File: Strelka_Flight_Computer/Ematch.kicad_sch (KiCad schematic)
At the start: 11 parts, among them Q10 AP2300, Q11 MMBT2222, Q9 AO3401A

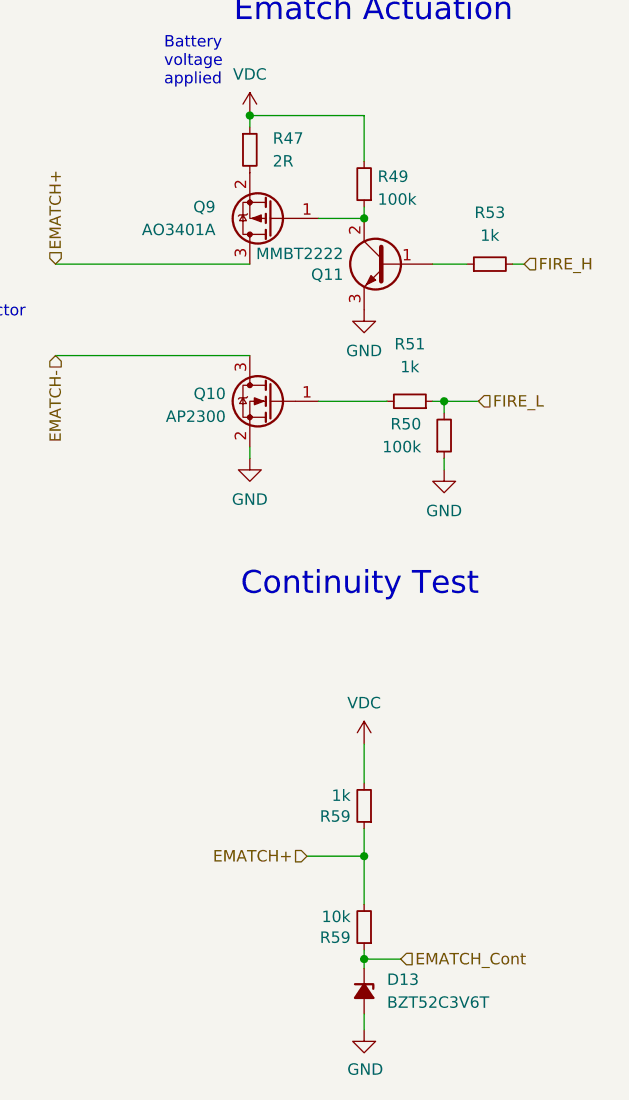
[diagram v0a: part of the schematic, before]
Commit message: Routing starting
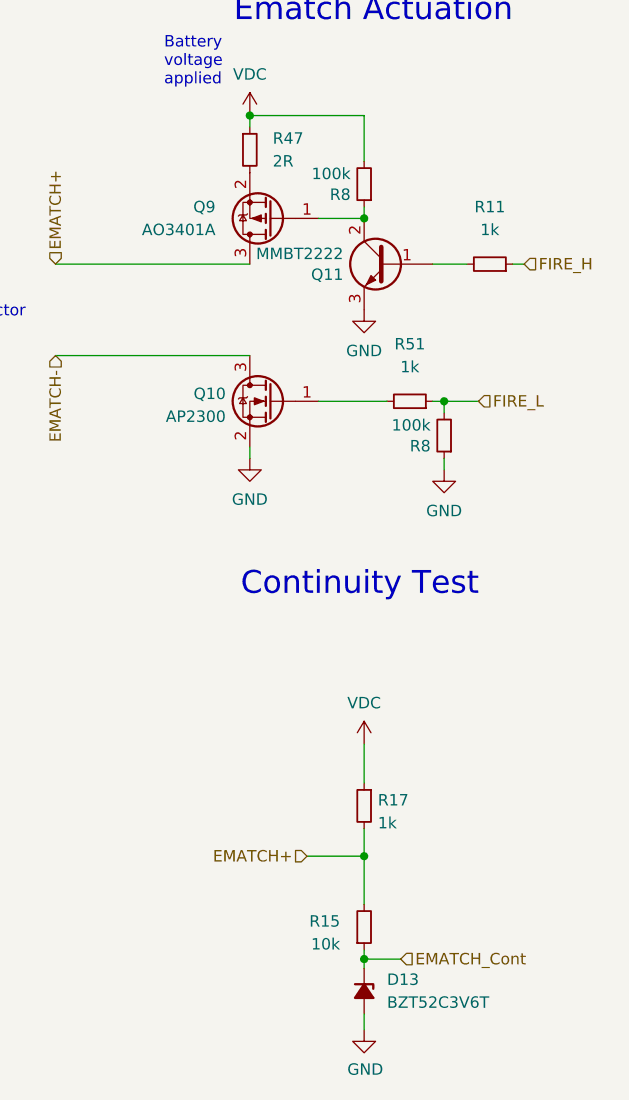
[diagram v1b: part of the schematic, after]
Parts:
- removed R49, R50: 100k, Resistor_SMD:R_0603_1608Metric, symbol Device:R_Small
- removed R53, R59: 1k, Resistor_SMD:R_0603_1608Metric, symbol Device:R_Small
- removed R59: 10k, Resistor_SMD:R_0603_1608Metric, symbol Device:R_Small
- added R11, R17: 1k, Resistor_SMD:R_0402_1005Metric, symbol Device:R_Small
- added R15: 10k, Resistor_SMD:R_0402_1005Metric, symbol Device:R_Small
- added R8 (x2): 100k, Resistor_SMD:R_0402_1005Metric, symbol Device:R_Small
- R51: footprint Resistor_SMD:R_0603_1608Metric -> Resistor_SMD:R_0402_1005Metric; LCSC (none) -> C11702
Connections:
- net EMATCH+: now also R15.2, R17.2
- net EMATCH_Cont: now also R15.1
- net FIRE_H: now also R11.1
- net FIRE_L: now also R8.2
- net GND: now also R8.1
- net VDC: now also R17.1, R8.2
- net at Q11.2 (C), Q9.1 (G): now also R8.1
- net at Q11.1 (B): now also R11.2

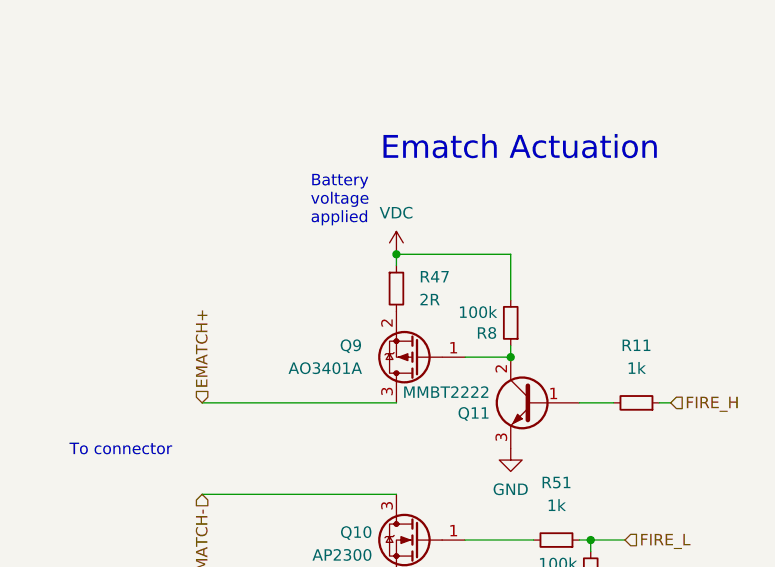
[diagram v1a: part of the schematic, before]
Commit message: Routing complete
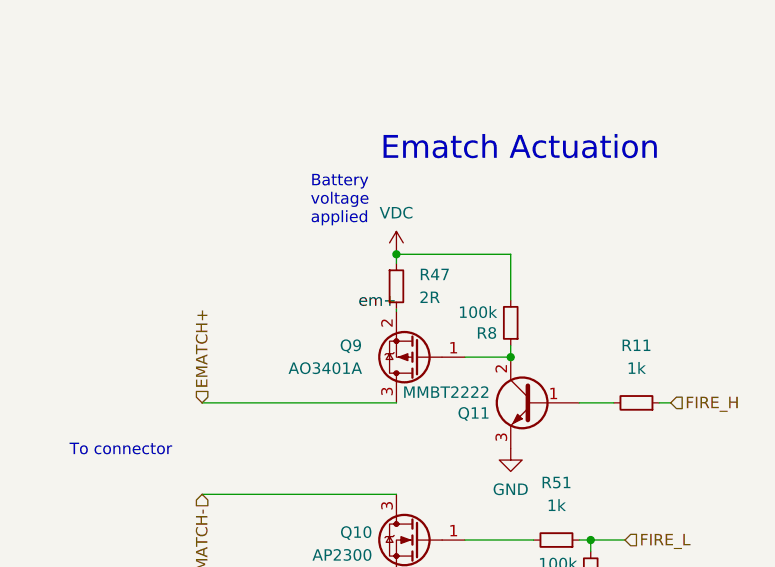
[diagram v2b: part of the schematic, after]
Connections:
- net em+: now reaches Q9.2 (S), R47.2
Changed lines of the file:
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@@
     (stroke (width 0) (type default))
   )
-  (wire (pts (xy 127 43.18) (xy 127 44.45))
+  (wire (pts (xy 127 49.276) (xy 127 49.53))
+    (stroke (width 0) (type default))
+  )
+  (wire (pts (xy 127 43.18) (xy 127 44.196))
     (stroke (width 0) (type default))
   )
@@
     (effects (font (size 2.54 2.54)) (justify left bottom))
   )
+  (label "em+" (at 127 49.403 180) (fields_autoplaced)
+    (effects (font (size 1.27 1.27)) (justify right bottom))
+  )
   (hierarchical_label "FIRE_H" (shape input) (at 157.48 59.69 0) (fields_autoplaced)
     (effects (font (size 1.27 1.27)) (justify left))
@@
     )
   )
-  (symbol (lib_id "Device:R_Small") (at 127 46.99 0) (unit 1)
-    (in_bom yes) (on_board yes) (dnp no) (fields_autoplaced)
-    (property "Reference" "R47" (at 129.54 45.7199 0)
-      (effects (font (size 1.27 1.27)) (justify left))
-    )
-    (property "Value" "2R" (at 129.54 48.2599 0)
-      (effects (font (size 1.27 1.27)) (justify left))
-    )
-    (property "Footprint" "Resistor_SMD:R_2512_6332Metric" (at 127 46.99 0)
-      (effects (font (size 1.27 1.27)) hide)
-    )
-    (property "Datasheet" "https://lcsc.com/product-detail/Chip-span-style-background-color-ff0-Resistor-span-Surface-Mount_UNI-ROYAL-Uniroyal-Elec-HP122WF200KT4E_C91926.html" (at 127 46.99 0)
-      (effects (font (size 1.27 1.27)) hide)
-    )
-    (property "LCSC#" "C91926" (at 127 46.99 0)
-      (effects (font (size 1.27 1.27)) hide)
-    )
+  (symbol (lib_id "Device:R_Small") (at 127 46.736 0) (unit 1)
+    (in_bom yes) (on_board yes) (dnp no) (fields_autoplaced)
+    (property "Reference" "R47" (at 129.54 45.4659 0)
+      (effects (font (size 1.27 1.27)) (justify left))
+    )
+    (property "Value" "2R" (at 129.54 48.0059 0)
+      (effects (font (size 1.27 1.27)) (justify left))
+    )
+    (property "Footprint" "Resistor_SMD:R_2512_6332Metric" (at 127 46.736 0)
+      (effects (font (size 1.27 1.27)) hide)
+    )
+    (property "Datasheet" "https://lcsc.com/product-detail/Chip-span-style-background-color-ff0-Resistor-span-Surface-Mount_UNI-ROYAL-Uniroyal-Elec-HP122WF200KT4E_C91926.html" (at 127 46.736 0)
+      (effects (font (size 1.27 1.27)) hide)
+    )
+    (property "LCSC#" "C91926" (at 127 46.736 0)
+      (effects (font (size 1.27 1.27)) hide)
+    )
